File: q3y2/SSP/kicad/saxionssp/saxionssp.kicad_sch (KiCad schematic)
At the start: 16 parts, among them Q1 Si2318CDS, Q2 Si2318CDS, U2 MPU-9250, U3 MPU-9250, U4 MPU-9250, U5 MPU-9250, U6 MPU-9250, U7 MPU-9250, U8 MAX17335X22+T

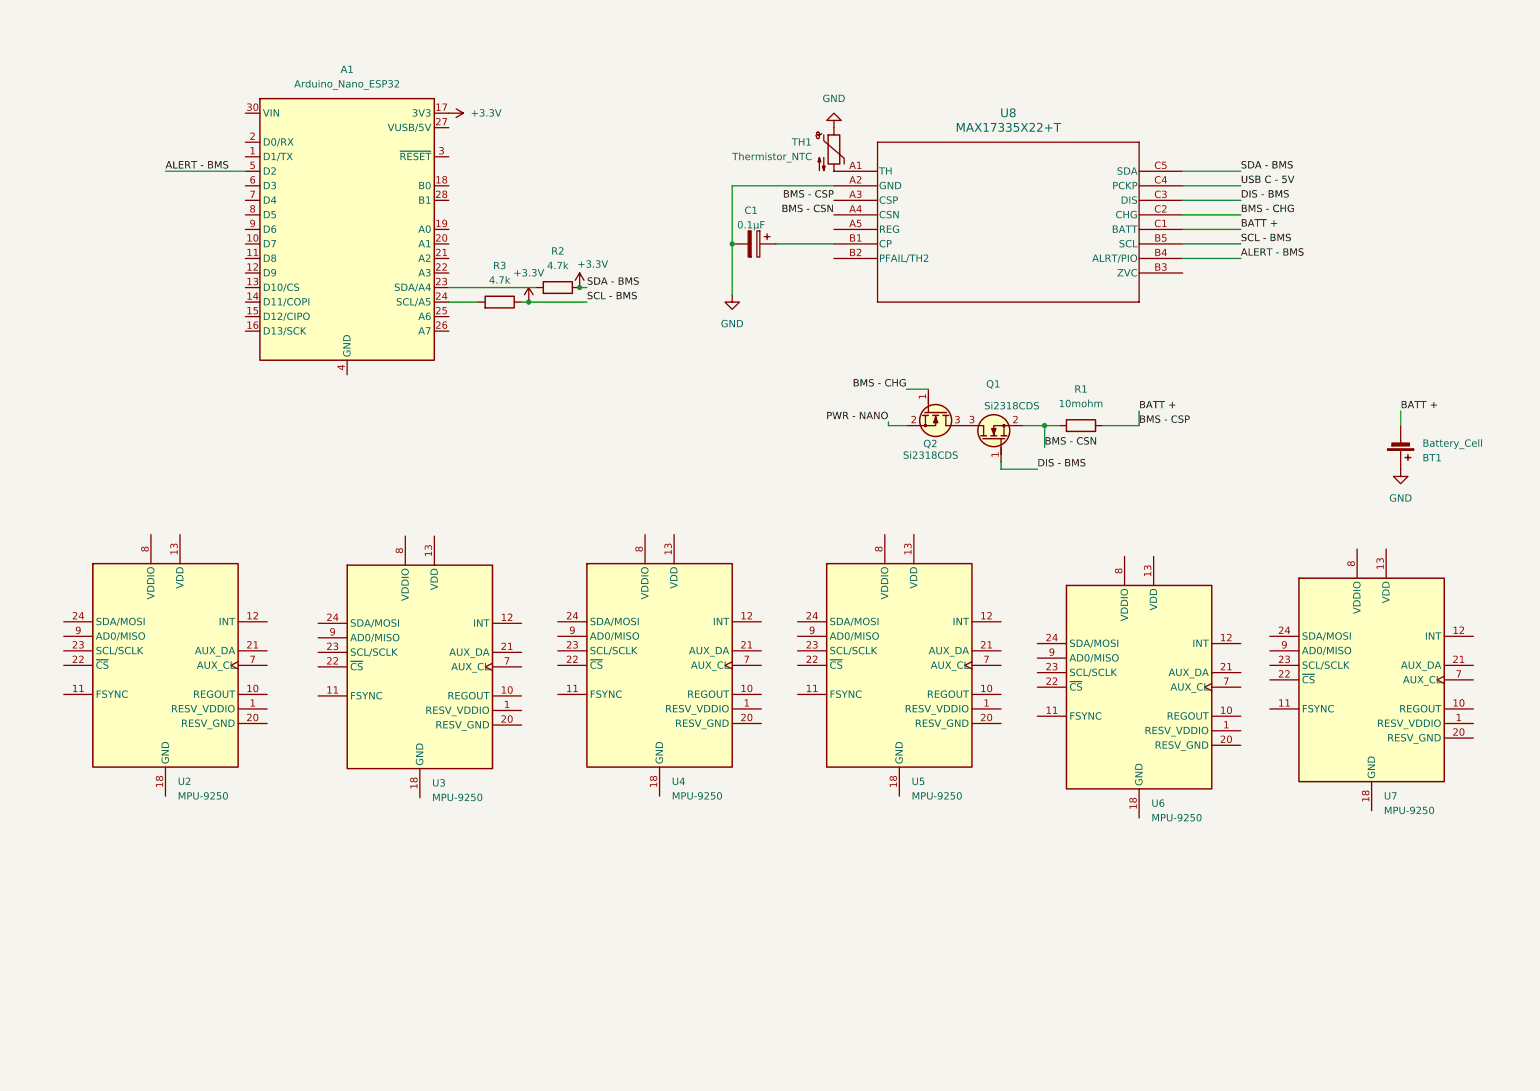
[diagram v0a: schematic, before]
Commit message: schematics ssp done
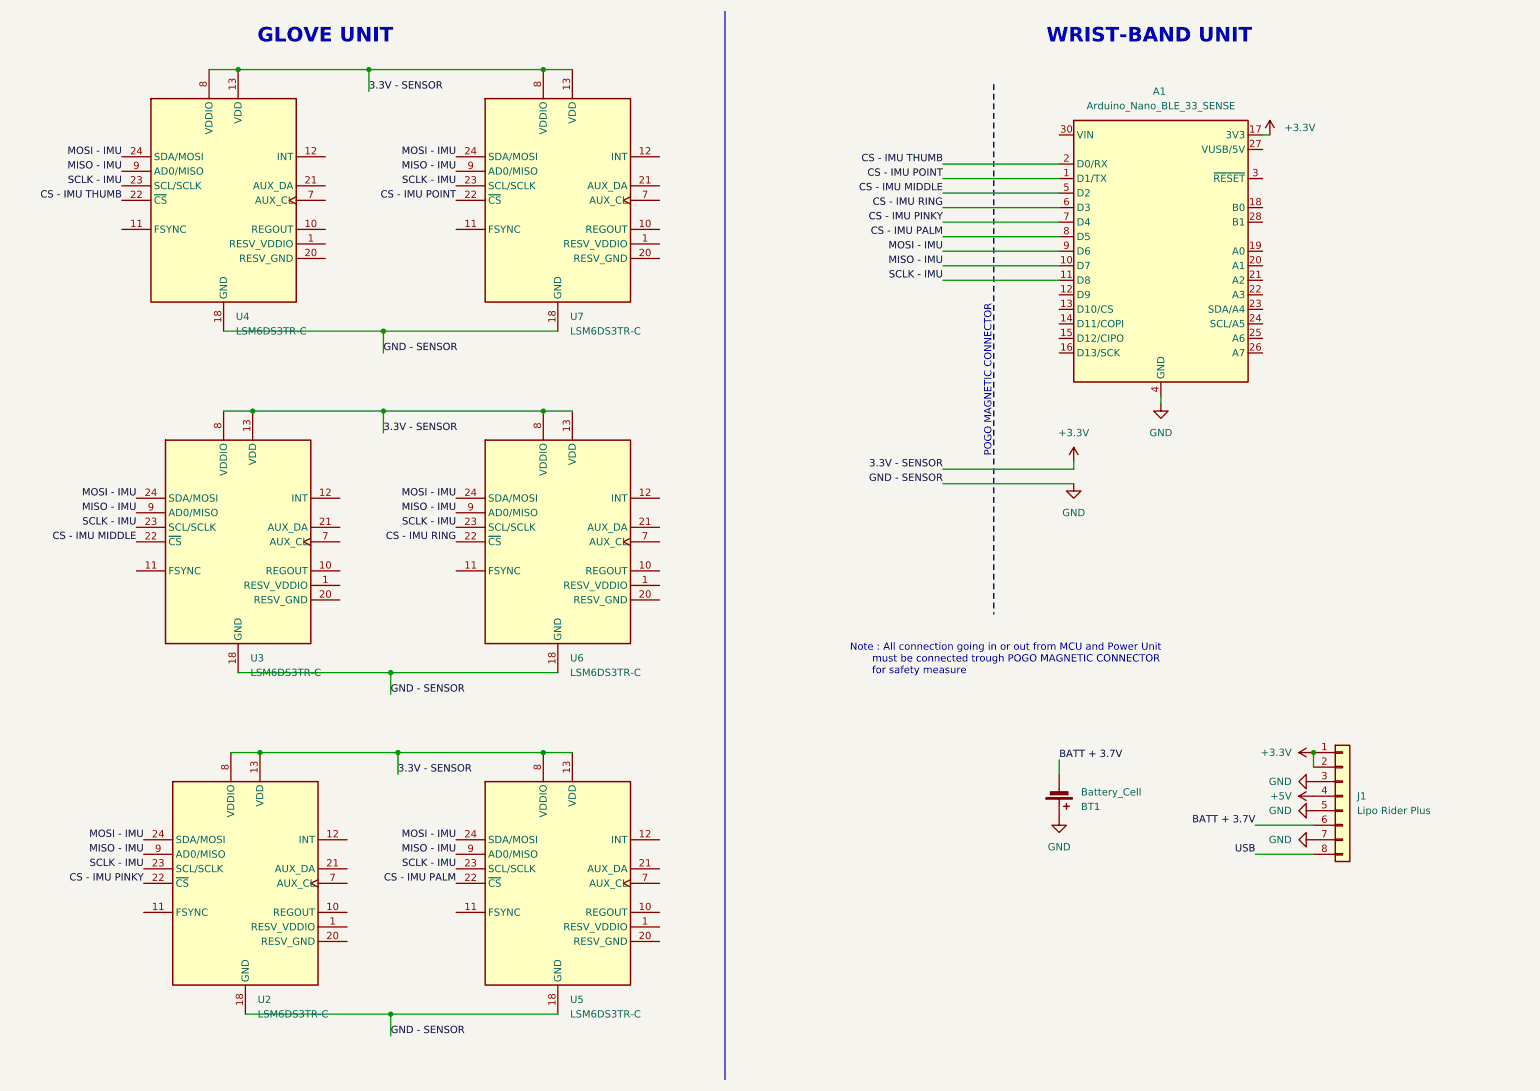
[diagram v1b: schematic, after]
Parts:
- removed C1: 0.1µF, PCM_Capacitor_SMD_AKL:CP_Elec_6.3x4.5, symbol PCM_Capacitor_AKL:CP_SMD_D6.3mm_H4.5mm
- removed Q1, Q2: Si2318CDS, PCM_Package_TO_SOT_SMD_AKL:SOT-23, symbol PCM_Transistor_MOSFET_AKL:Si2318CDS
- removed R1: 10mohm, PCM_Resistor_SMD_AKL:R_1206_3216Metric, symbol PCM_Resistor_AKL:R_1206
- removed R2, R3: 4.7k, PCM_Resistor_SMD_AKL:R_1206_3216Metric, symbol PCM_Resistor_AKL:R_1206
- removed TH1: Thermistor_NTC, symbol Device:Thermistor_NTC
- removed U8: MAX17335X22+T, 21-100433_W151J2+1_ADI:21-100433_W151J2&plus_1_ADI, symbol MAX17335X22:MAX17335X22+T
- added J1: Lipo Rider Plus, symbol Connector_Generic:Conn_01x08
- A1: value Arduino_Nano_ESP32 -> Arduino_Nano_BLE_33_SENSE
- U2, U3, U4, U5, U6, U7: value MPU-9250 -> LSM6DS3TR-C
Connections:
- net ALERT - BMS is gone; now on net CS - IMU MIDDLE: A1.5 (D2)
- net +3.3V: now also U2.13 (VDD), U2.8 (VDDIO), U3.13 (VDD), U3.8 (VDDIO), U4.13 (VDD), U4.8 (VDDIO), U5.13 (VDD), U5.8 (VDDIO), U6.13 (VDD), U6.8 (VDDIO), U7.13 (VDD), U7.8 (VDDIO), J1.1 (Pin_1), J1.2 (Pin_2)
- net GND: now also A1.29 (GND), A1.4 (GND), U2.18 (GND), U3.18 (GND), U4.18 (GND), U5.18 (GND), U6.18 (GND), U7.18 (GND), J1.3 (Pin_3), J1.5 (Pin_5), J1.7 (Pin_7)
- net CS - IMU THUMB: now reaches U4.22 (~{CS})
- net CS - IMU THUMB: now also A1.2 (D0/RX)
- net SCLK - IMU: now reaches U4.23 (SCL/SCLK)
- net SCLK - IMU: now also A1.11 (D8), U2.23 (SCL/SCLK), U3.23 (SCL/SCLK), U5.23 (SCL/SCLK), U6.23 (SCL/SCLK), U7.23 (SCL/SCLK)
- net MOSI - IMU: now reaches U4.24 (SDA/MOSI)
- net MOSI - IMU: now also A1.9 (D6), U2.24 (SDA/MOSI), U3.24 (SDA/MOSI), U5.24 (SDA/MOSI), U6.24 (SDA/MOSI), U7.24 (SDA/MOSI)
- net MISO - IMU: now reaches U4.9 (AD0/MISO)
- net MISO - IMU: now also A1.10 (D7), U2.9 (AD0/MISO), U3.9 (AD0/MISO), U5.9 (AD0/MISO), U6.9 (AD0/MISO), U7.9 (AD0/MISO)
- net CS - IMU MIDDLE: now reaches U3.22 (~{CS})
- net CS - IMU POINT: now reaches U7.22 (~{CS})
- net CS - IMU POINT: now also A1.1 (D1/TX)
- net CS - IMU RING: now reaches U6.22 (~{CS})
- net CS - IMU RING: now also A1.6 (D3)
- net CS - IMU PINKY: now reaches U2.22 (~{CS})
- net CS - IMU PINKY: now also A1.7 (D4)
- net CS - IMU PALM: now reaches U5.22 (~{CS})
- net CS - IMU PALM: now also A1.8 (D5)
- net BATT + renamed BATT + 3.7V
- net BATT + 3.7V: now also J1.6 (Pin_6)
- new net +5V: J1.4 (Pin_4)
- new net USB: J1.8 (Pin_8)
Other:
- note added: "GLOVE UNIT"
- note added: "Note : All connection going in or out from MCU and Power Unit must be connected trough POGO MAGNETIC CONNECTOR for safety measure"
- note added: "POGO MAGNETIC CONNECTOR"
- note added: "WRIST-BAND UNIT"
- company: (none) -> SAXION PROJECT GESTURED 
- title: (none) -> WEARABLE UNIT SPI CONNECTION
- moved on the sheet: A1, BT1

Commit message: add ssp
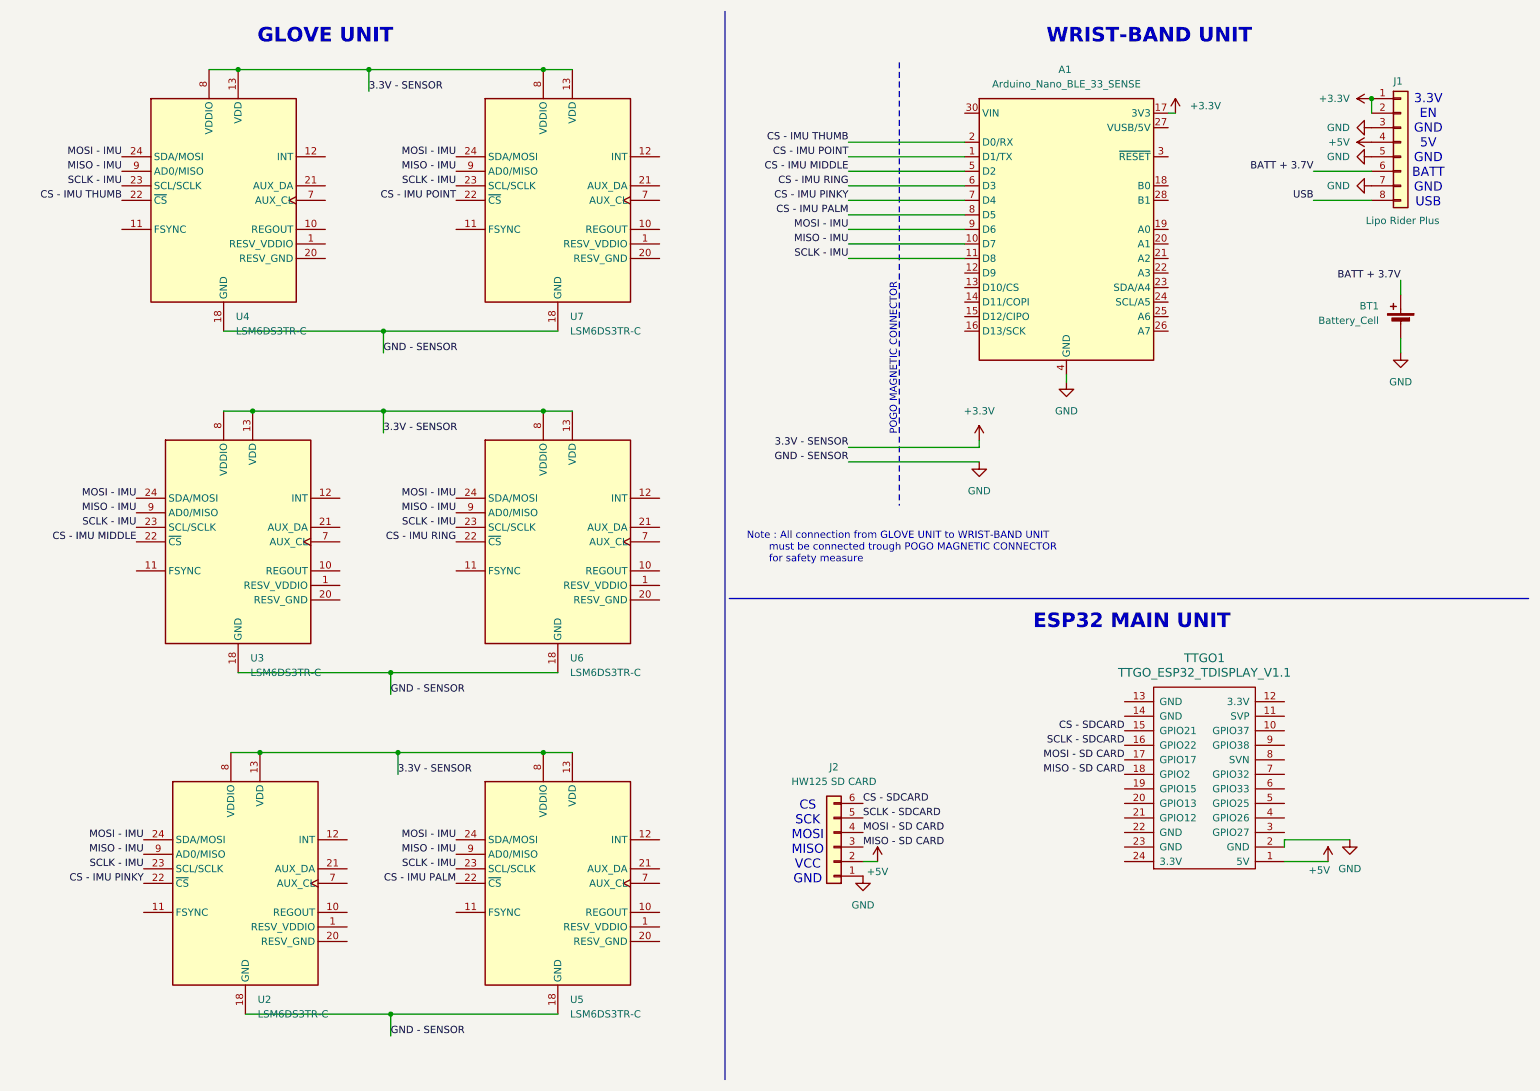
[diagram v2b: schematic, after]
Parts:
- added J2: HW125 SD CARD, symbol Connector_Generic:Conn_01x06
- added TTGO1: TTGO_ESP32_TDISPLAY_V1.1, ttgo-tdisplay-kicad-master:TTGO_ESP32_TDisplay_v1.1, symbol ttgo_esp32:TTGO_ESP32_TDISPLAY_V1.1
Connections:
- net +5V: now also J2.2 (Pin_2), TTGO1.1 (5V)
- net BATT + 3.7V: now also BT1.1 (+); no longer BT1.2 (-)
- net GND: now also BT1.2 (-), J2.1 (Pin_1), TTGO1.2 (GND); no longer BT1.1 (+)
- new net CS - SDCARD: J2.6 (Pin_6), TTGO1.15 (GPIO21)
- new net MISO - SD CARD: J2.3 (Pin_3), TTGO1.18 (GPIO2)
- new net MOSI - SD CARD: J2.4 (Pin_4), TTGO1.17 (GPIO17)
- new net SCLK - SDCARD: J2.5 (Pin_5), TTGO1.16 (GPIO22)
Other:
- note added: "3.3V EN GND 5V GND BATT GND USB"
- note added: "CS SCK MOSI MISO VCC GND"
- note added: "ESP32 MAIN UNIT"
- note added: "Note : All connection from GLOVE UNIT to WRIST-BAND UNIT must be connected trough POGO MAGNETIC CONNECTOR for safety measure"
- note removed: "Note : All connection going in or out from MCU and Power Unit must be connected trough POGO MAGNETIC CONNECTOR for safety measure"
- company: SAXION PROJECT GESTURED  -> SAXION UNIVERSITY OF APPLIED SCIENCE
- title: WEARABLE UNIT SPI CONNECTION -> GESTURED CONTROL SMART DEVICE
- moved on the sheet: A1, BT1, J1
